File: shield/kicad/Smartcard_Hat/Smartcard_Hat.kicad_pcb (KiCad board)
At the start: 2 copper layers, 68.6 x 53.3 mm, 43 parts, among them J10 SFV12R-2STE1HLF, J8 7712P0225A25LF, U6 ST8034HNQR

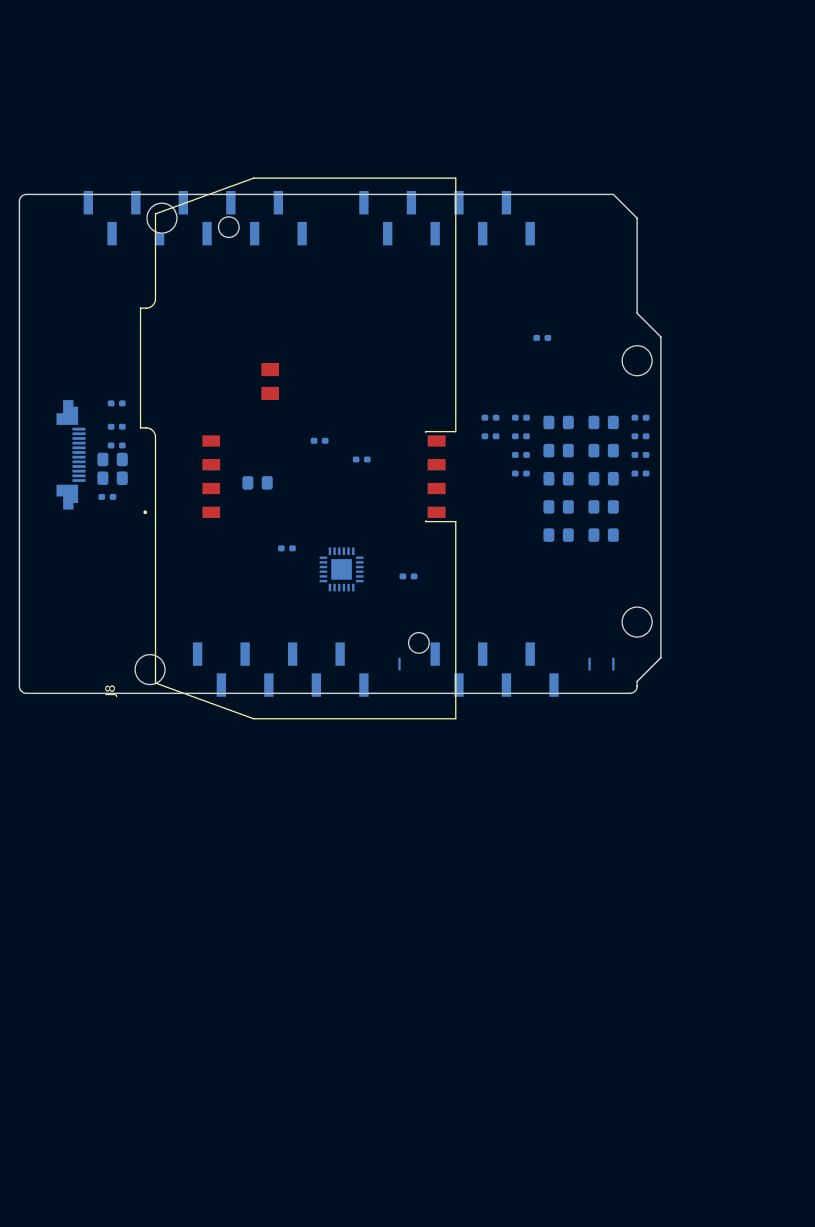
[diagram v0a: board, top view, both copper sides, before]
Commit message: wip
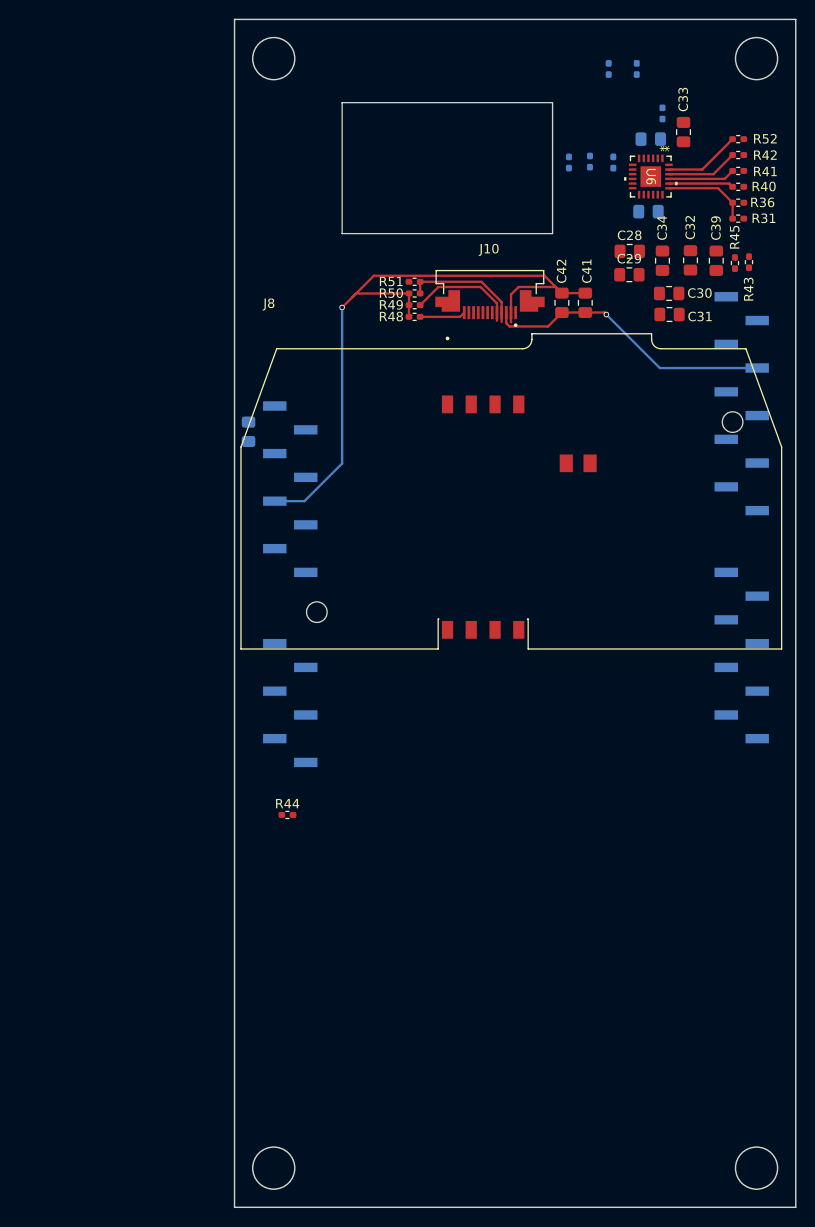
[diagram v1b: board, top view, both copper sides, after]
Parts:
- removed MH1, MH2, MH3, MH4: MountingHole_3.2mm, Arduino_MountingHole:MountingHole_3.2mm
- C28, C29, C30, C31, C32, C33, C34, C39, C41, C42, J10, R31, R36, R40, R41, R42, R43, R44, R45, R48, R49, R50, R51, R52: moved to F.Cu
- J11: footprint Connector_PinHeader_2.54mm:PinHeader_1x10_P2.54mm_Vertical_SMD_Pin1Left -> Connector_PinHeader_2.54mm:PinHeader_1x10_P2.54mm_Vertical_SMD_Pin1Right
- J12, J9: footprint Connector_PinHeader_2.54mm:PinHeader_1x08_P2.54mm_Vertical_SMD_Pin1Left -> Connector_PinHeader_2.54mm:PinHeader_1x08_P2.54mm_Vertical_SMD_Pin1Right
- J13: footprint Connector_PinHeader_2.54mm:PinHeader_1x06_P2.54mm_Vertical_SMD_Pin1Left -> Connector_PinHeader_2.54mm:PinHeader_1x06_P2.54mm_Vertical_SMD_Pin1Right
- J8: footprint 7312P0225A13LF:AMPHENOL_7312P0225A13LF -> Library:AMPHENOL_7312P0225A13LF
- U6: footprint footprints:QFN24_4x4x0.8_STM -> Library:QFN24_4x4x0.8_STM; moved to F.Cu
- moved J11 61.7 mm to (177.2, 69.0), turned to 0 degrees
- moved R43 58.1 mm to (178.0, 53.9), turned to 90 degrees
- moved R44 56.8 mm to (128.7, 113.0), turned to 0 degrees
- moved J12 56.4 mm to (177.2, 96.0), turned to 0 degrees
- moved U6 53.4 mm to (167.5, 44.8), turned to -90 degrees
- moved R41 53.2 mm to (176.8, 44.1)
- moved C41 53.2 mm to (160.5, 58.2), turned to -90 degrees
- moved R42 51.8 mm to (176.8, 42.5), turned to 180 degrees
- moved C42 51.6 mm to (158.0, 58.2), turned to -90 degrees
- moved J10 49.6 mm to (150.3, 56.9), turned to 180 degrees
- moved R35 49.4 mm to (163.5, 43.2), turned to -90 degrees
- moved R46 41.4 mm to (163.0, 33.2), turned to 90 degrees
- moved R32 41.2 mm to (166.0, 33.2), turned to 90 degrees
- moved R50 39.4 mm to (142.2, 57.2), turned to 0 degrees
- moved R47 38.6 mm to (168.8, 38.0), turned to -90 degrees
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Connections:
- J10 pad 12: /QR_Scanner/QR_TRIG -> QR_TRIG
- J10 pad 5: /QR_Scanner/QR_UART_TX -> QR_UART_TX
- J10 pad 9: /QR_Scanner/QR_BEEP -> UC_BEEP
- J11 pad 1: /STM32F469I-DISCO-Interface/SC_RST -> SC_RST
- J11 pad 2: /STM32F469I-DISCO-Interface/SC_AUX2 -> SC_AUX2
- J12 pad 1: /STM32F469I-DISCO-Interface/QR_UART_TX -> QR_UART_TX
- J12 pad 2: /STM32F469I-DISCO-Interface/QR_UART_RX -> QR_UART_RX
- J12 pad 3: /STM32F469I-DISCO-Interface/QR_TRIG -> QR_TRIG
- J12 pad 4: /STM32F469I-DISCO-Interface/UC_BEEP -> UC_BEEP
- J12 pad 5: /STM32F469I-DISCO-Interface/SC_CLKDIV2 -> SC_CLKDIV2
- J12 pad 6: /STM32F469I-DISCO-Interface/SC_IO -> SC_IO
- J12 pad 7: /STM32F469I-DISCO-Interface/SC_AUX1 -> SC_AUX1
- J12 pad 8: /STM32F469I-DISCO-Interface/SC_CLKDIV1 -> SC_CLKDIV1
- J13 pad 2: /STM32F469I-DISCO-Interface/SC_nOFF -> SC_nOFF
- J13 pad 3: /STM32F469I-DISCO-Interface/SC_VCC_SEL1 -> SC_VCC_SEL1
- J13 pad 4: /STM32F469I-DISCO-Interface/SC_VCC_SEL2 -> SC_VCC_SEL2
- J13 pad 5: /STM32F469I-DISCO-Interface/SC_nCMDVCC -> SC_nCMDVCC
- J13 pad 6: /STM32F469I-DISCO-Interface/SC_CLK -> SC_CLK
- R31 pad 2: /SmartCard_Reader/SC_nOFF -> Net-(U6-*OFF)
- R32 pad 2: /SmartCard_Reader/SC_CLKDIV1 -> SC_CLKDIV1
- R33 pad 2: /SmartCard_Reader/SC_VCC_SEL2 -> SC_VCC_SEL2
- R34 pad 2: /SmartCard_Reader/SC_VCC_SEL1 -> SC_VCC_SEL1
- R35 pad 2: Net-(U6-*CMDVCC) -> SC_nCMDVCC
- R36 pad 1: /SmartCard_Reader/SC_nCMDVCC -> SC_nOFF
- R36 pad 2: Net-(U6-*CMDVCC) -> Net-(U6-*OFF)
- R40 pad 1: /SmartCard_Reader/SC_IO -> SC_IO
- R41 pad 1: /SmartCard_Reader/SC_AUX1 -> SC_AUX1
- R42 pad 1: /SmartCard_Reader/SC_AUX2 -> SC_AUX2
- R44 pad 1: /SmartCard_Reader/SC_CLK -> SC_CLK
- R46 pad 1: /SmartCard_Reader/SC_CLKDIV2 -> SC_CLKDIV2
- R47 pad 1: /SmartCard_Reader/SC_RST -> SC_RST
- R48 pad 2: /QR_Scanner/QR_TRIG -> QR_TRIG
- R49 pad 2: /QR_Scanner/QR_UART_TX -> QR_UART_TX
- R51 pad 1: /QR_Scanner/QR_UART_RX -> QR_UART_RX
- U6 pad 19: /SmartCard_Reader/SC_nOFF -> Net-(U6-*OFF)
- U6 pad 2: /SmartCard_Reader/SC_VCC_SEL2 -> SC_VCC_SEL2
- U6 pad 3: /SmartCard_Reader/SC_RST -> SC_RST
- U6 pad 4: /SmartCard_Reader/SC_VCC_SEL1 -> SC_VCC_SEL1
- U6 pad 5: Net-(U6-*CMDVCC) -> SC_nCMDVCC
- U6 pad 6: /SmartCard_Reader/SC_CLKDIV1 -> SC_CLKDIV1
- U6 pad 7: /SmartCard_Reader/SC_CLKDIV2 -> SC_CLKDIV2
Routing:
- net +3V3: track 0.00 -> 71.4 mm, vias 0 -> 1
- net GND: track 1.18 -> 31.2 mm, vias 0 -> 1
- net Net-(J10-Pad4): track 0.00 -> 13.0 mm
- net QR_UART_TX: track 0.00 -> 11.6 mm
- net Net-(U6-*OFF): track 0.00 -> 9.15 mm
- net Net-(U6-XTAL1): track 0.00 -> 8.15 mm
- net Net-(U6-AUXUC2): track 0.00 -> 7.66 mm
- net Net-(U6-AUXUC1): track 0.00 -> 7.16 mm
- net Net-(U6-I/OUC): track 0.00 -> 6.95 mm
- net QR_TRIG: track 0.00 -> 4.89 mm
- net (no net): track 2.35 -> 0.00 mm
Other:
- board size 68.6 x 53.3 mm -> 60 x 127 mm
